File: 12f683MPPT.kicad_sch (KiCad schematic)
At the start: 50 parts, among them J1 Conn_01x01_Male, J2 Conn_01x01_Male, J3 Conn_01x01_Male, J4 Conn_01x01_Male, J5 Vin, J6 GND, J7 12V, Q1 BUK9511-55A127, Q2 BUK9511-55A127, Q3 2N2222A, Q4 2N2222A, Q5 2N2907A, SW1 SW_Push, U1 LM7805_TO220, U2 PIC12F683-IP, U3 LM358

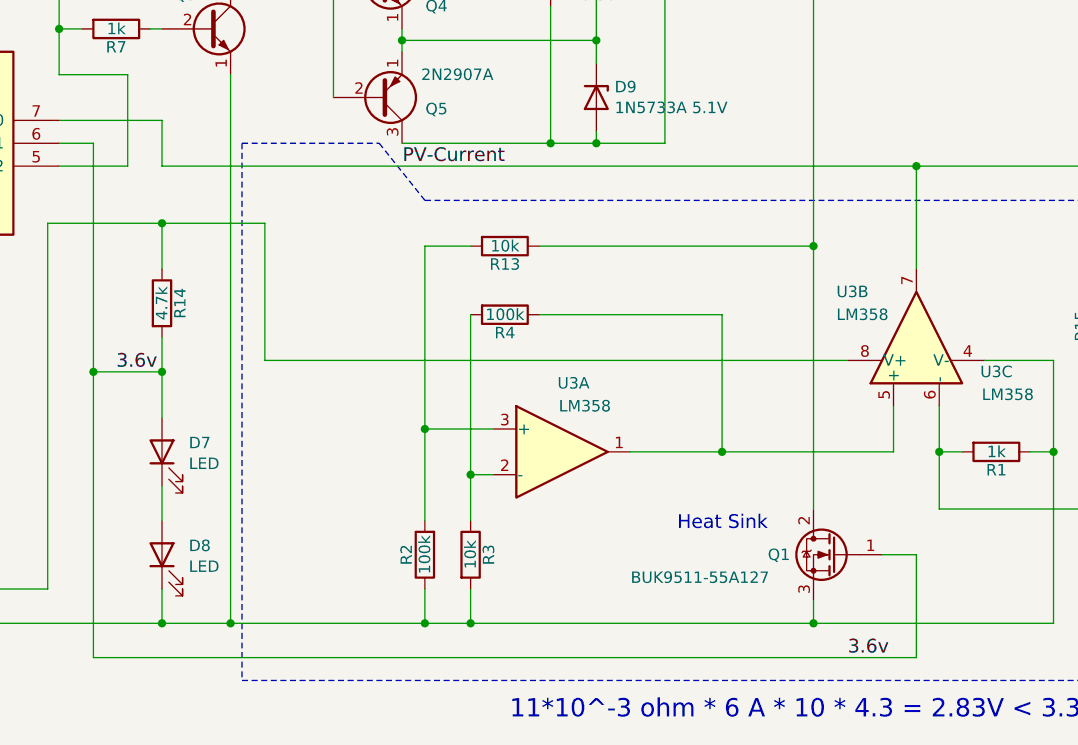
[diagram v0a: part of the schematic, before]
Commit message: Revert "Remove C5 capacitor."
This reverts commit 91564baa6f44f8037db3e26806d1f3bf7336a2bb.
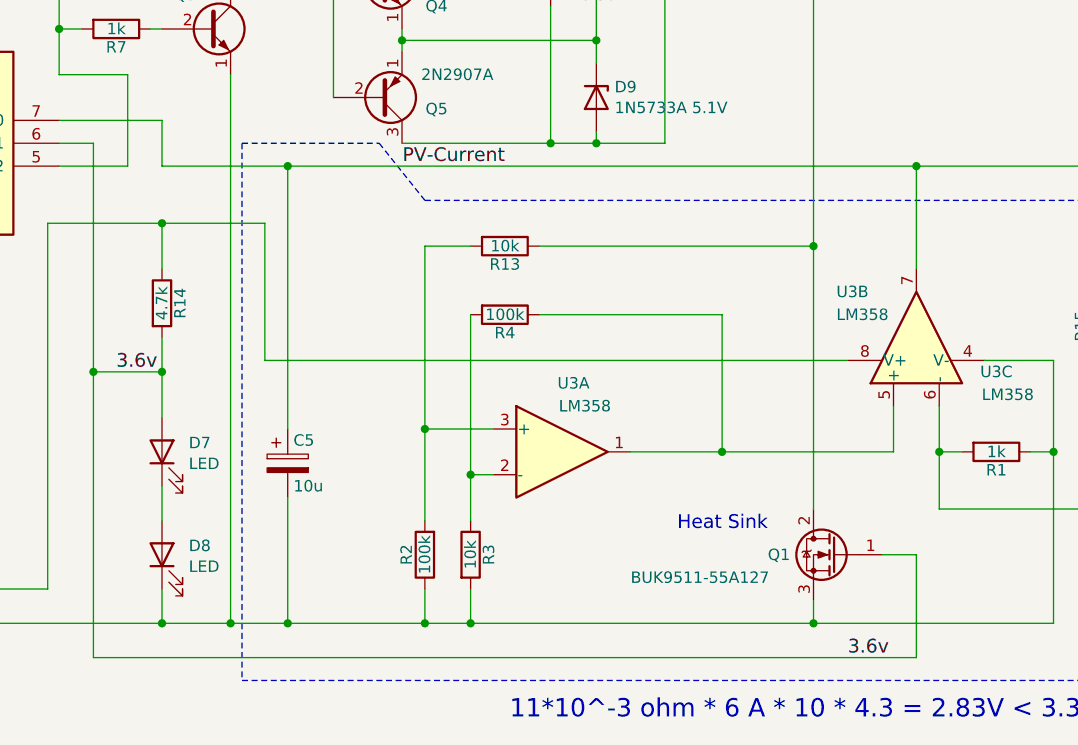
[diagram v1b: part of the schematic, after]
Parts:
- added C5: 10u, Capacitor_THT:CP_Radial_D8.0mm_P2.50mm, symbol Device:CP
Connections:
- net GNDPWR: now also C5.2
- net PV-Current: now also C5.1
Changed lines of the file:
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@@
 	)
 	(junction
+		(at 154.94 91.44)
+		(diameter 0)
+		(color 0 0 0 0)
+	)
+	(junction
 		(at 54.61 55.88)
 		(diameter 0)
@@
 	)
 	(junction
+		(at 154.94 142.24)
+		(diameter 0)
+		(color 0 0 0 0)
+	)
+	(junction
 		(at 224.79 91.44)
 		(diameter 0)
@@
 	(wire
 		(pts
+			(xy 154.94 91.44) (xy 224.79 91.44)
+		)
+		(stroke
+			(width 0)
+			(type default)
+		)
+	)
+	(wire
+		(pts
 			(xy 129.54 88.9) (xy 133.35 88.9)
 		)
@@
 	(wire
 		(pts
-			(xy 140.97 91.44) (xy 224.79 91.44)
+			(xy 154.94 91.44) (xy 140.97 91.44)
 		)
 		(stroke
@@
 	(wire
 		(pts
+			(xy 154.94 128.27) (xy 154.94 142.24)
+		)
+		(stroke
+			(width 0)
+			(type default)
+		)
+	)
+	(wire
+		(pts
 			(xy 224.79 146.05) (xy 224.79 134.62)
 		)
@@
 	(wire
 		(pts
-			(xy 148.59 142.24) (xy 170.18 142.24)
+			(xy 154.94 142.24) (xy 148.59 142.24)
+		)
+		(stroke
+			(width 0)
+			(type default)
+		)
+	)
+	(wire
+		(pts
+			(xy 170.18 142.24) (xy 154.94 142.24)
 		)
 		(stroke
@@
 	(wire
 		(pts
+			(xy 154.94 120.65) (xy 154.94 91.44)
+		)
+		(stroke
+			(width 0)
+			(type default)
+		)
+	)
+	(wire
+		(pts
 			(xy 83.82 55.88) (xy 82.55 55.88)
 		)
@@
 					(unit 1)
 				)
+			)
+		)
+	)
+	(symbol
+		(lib_id "Device:CP")
+		(at 154.94 124.46 0)
+		(unit 1)
+		(exclude_from_sim no)
+		(in_bom yes)
+		(on_board yes)
+		(dnp no)
+		(property "Reference" "C5"
+			(at 155.575 121.92 0)
+			(effects
+				(font
+					(size 1.27 1.27)
+				)
+				(justify left)
+			)
+		)
+		(property "Value" "10u"
+			(at 155.575 127 0)
+			(effects
+				(font
+					(size 1.27 1.27)
+				)
+				(justify left)
+			)
+		)
+		(property "Footprint" "Capacitor_THT:CP_Radial_D8.0mm_P2.50mm"
+			(at 155.9052 128.27 0)
+			(effects
+				(font
+					(size 0.762 0.762)
+				)
+				(hide yes)
+			)
+		)
+		(property "Datasheet" ""
+			(at 154.94 124.46 0)
+			(effects
+				(font
+					(size 1.524 1.524)
+				)
+			)
+		)
+		(property "Description" ""
+			(at 154.94 124.46 0)
+			(effects
+				(font
+					(size 1.27 1.27)
+				)
+			)
+		)
+		(pin "1"
+		)
+		(pin "2"
+		)
+		(instances
+			(project ""
+				(path "/c54864ce-ba59-4422-a8c7-824cf583dfc9"
+					(reference "C5")
+					(unit 1)
+				)
